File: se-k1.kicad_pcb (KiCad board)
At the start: 2 copper layers, 100 x 70 mm, 42 parts, among them J1 USB_C_Receptacle_USB2.0_14P, M1 MountingHole_2.7mm_M2.5, M2 MountingHole_2.7mm_M2.5, M3 MountingHole_2.7mm_M2.5, M4 MountingHole_2.7mm_M2.5, U1 ESP32-S3-MINI-1U, U3 W25Q16JVSSIQ, U4 AMS1117-3.3

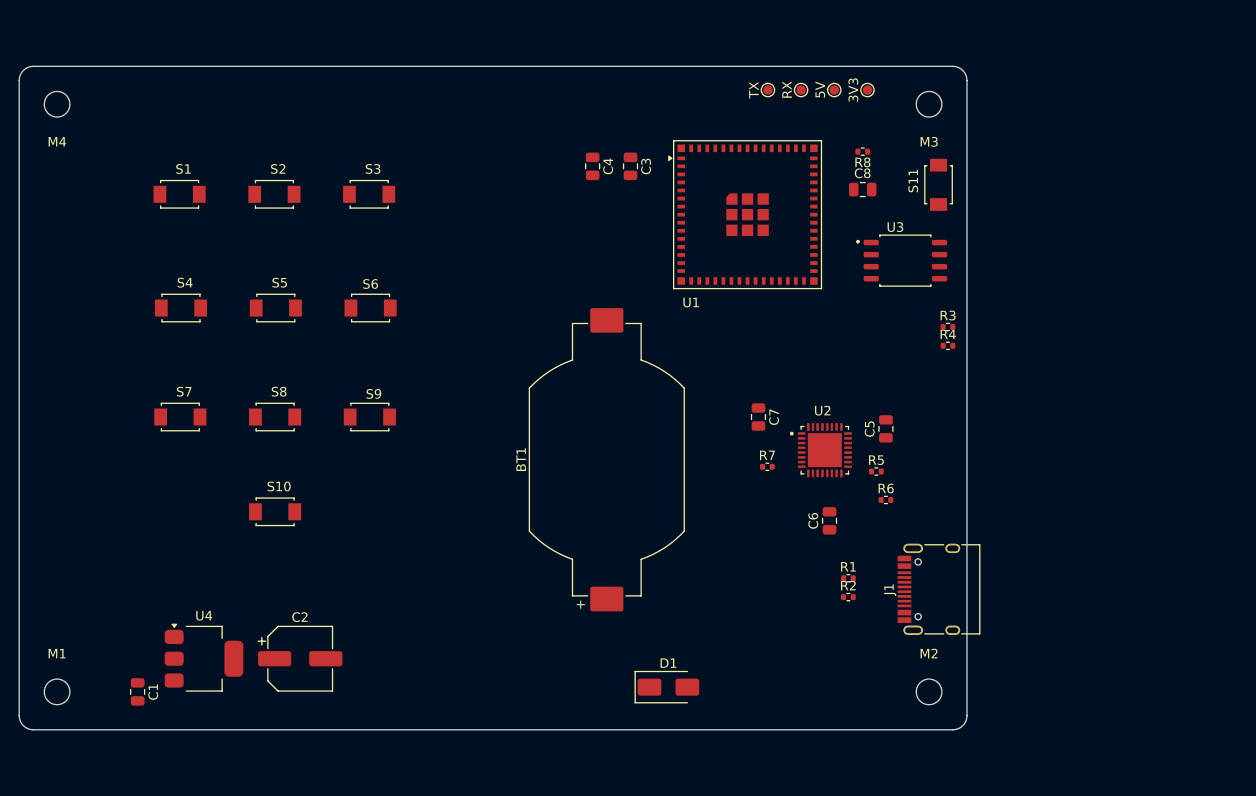
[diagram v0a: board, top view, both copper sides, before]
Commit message: finish!
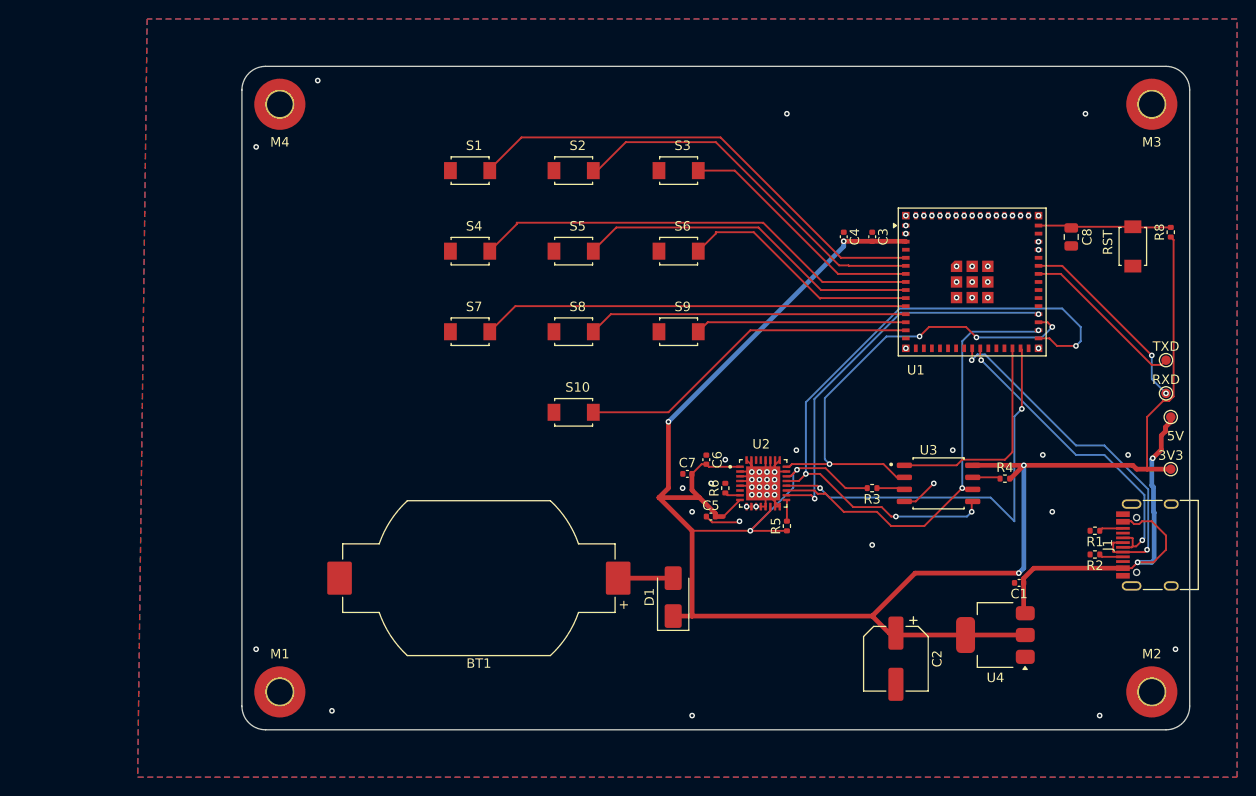
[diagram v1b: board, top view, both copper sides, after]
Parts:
- removed R7: 10k, Resistor_SMD:R_0402_1005Metric
- removed RX: RX, TestPoint:TestPoint_Pad_D1.0mm
- removed S11: TS-1088-AR02016, TS-1088-AR02016:SW_TS-1088-AR02016
- removed TX: TX, TestPoint:TestPoint_Pad_D1.0mm
- added RST: TS-1088-AR02016, TS-1088-AR02016:SW_TS-1088-AR02016, F.Cu at (194.0, 69.0)
- added RXD: RX, TestPoint:TestPoint_Pad_D1.0mm, F.Cu at (197.5, 84.5)
- added TXD: TX, TestPoint:TestPoint_Pad_D1.0mm, F.Cu at (197.5, 81.0)
- C1, C3, C4, C5, C6: footprint Capacitor_SMD:C_0805_2012Metric -> Capacitor_SMD:C_0402_1005Metric
- C7: value 100nF -> 10uF; footprint Capacitor_SMD:C_0805_2012Metric -> Capacitor_SMD:C_0402_1005Metric
- M1, M2, M3, M4: value MountingHole_2.7mm_M2.5 -> MountingHole_2.7mm_M2.5_Pad_TopOnly; footprint MountingHole:MountingHole_2.7mm_M2.5 -> MountingHole:MountingHole_2.7mm_M2.5_Pad_TopOnly
- U2: value ~ -> SLM9670AQ20FW1311XTMA1; footprint SLB9670VQ20FW785XUMA1:QFN50P500X500X90-33N -> SLM9670AQ20FW1311XTMA1:QFN50P500X500X90-33N
- moved C1 93.7 mm to (182.0, 104.5), turned to 180 degrees
- moved U4 83.5 mm to (179.5, 110.0), turned to 180 degrees
- moved C2 62.8 mm to (169.0, 112.5), turned to -90 degrees
- moved 3V3 51.2 mm to (198.0, 92.5), turned to 0 degrees
- moved 5V 49.5 mm to (198.0, 87.0), turned to 0 degrees
- moved S9 33.8 mm to (146.1, 78.0)
- moved R8 33.6 mm to (198.0, 67.5), turned to 90 degrees
- moved S10 33.2 mm to (135.0, 86.5)
- moved S6 33.0 mm to (146.1, 69.5)
- moved S8 32.8 mm to (135.0, 78.0)
- moved S3 32.7 mm to (146.1, 61.0)
- moved S5 32.0 mm to (135.0, 69.5)
- moved S7 31.9 mm to (124.1, 78.0)
- moved S2 31.7 mm to (135.0, 61.0)
- moved S4 31.1 mm to (124.1, 69.5)
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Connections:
- C5 pad 1: +3V3 -> GND
- C5 pad 2: GND -> +3V3
- R5 pad 1: /TPM_PIRQ -> +3V3
- R5 pad 2: +3V3 -> Net-(U2-~{RST})
- R6 pad 1: Net-(U2-RST) -> Net-(U2-PP)
- R6 pad 2: +3V3 -> GND
- S2 pad 2: /B4 -> /B2
- S3 pad 2: /B7 -> /B3
- S6 pad 2: /B8 -> /B6
- S7 pad 2: /B3 -> /B7
- S8 pad 2: /B6 -> /B8
- U2 pad 10: unconnected-(U2-NC-Pad10) -> GND
- U2 pad 11: unconnected-(U2-NC-Pad11) -> GND
- U2 pad 12: unconnected-(U2-NC-Pad12) -> GND
- U2 pad 13: unconnected-(U2-NC-Pad13) -> GND
- U2 pad 15: unconnected-(U2-NC-Pad15) -> GND
- U2 pad 17: Net-(U2-RST) -> Net-(U2-~{RST})
- U2 pad 25: unconnected-(U2-NC-Pad25) -> GND
- U2 pad 26: unconnected-(U2-NC-Pad26) -> GND
- U2 pad 27: unconnected-(U2-NC-Pad27) -> GND
- U2 pad 28: unconnected-(U2-NC-Pad28) -> GND
- U2 pad 29: unconnected-(U2-NC-Pad29) -> (no net)
- U2 pad 3: unconnected-(U2-NC-Pad3) -> GND
- U2 pad 30: unconnected-(U2-NC-Pad30) -> (no net)
- U2 pad 31: unconnected-(U2-NC-Pad31) -> GND
- U2 pad 33: (no net) -> GND
- U2 pad 4: unconnected-(U2-NC-Pad4) -> GND
- U2 pad 5: unconnected-(U2-NC-Pad5) -> GND
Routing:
- net +3V3: track 0.00 -> 222.2 mm, vias 0 -> 6
- net /MOSI: track 0.00 -> 71.0 mm, vias 0 -> 4
- net /B1: track 0.00 -> 50.7 mm
- net /MISO: track 0.00 -> 50.0 mm, vias 0 -> 4
- net /B4: track 0.00 -> 47.8 mm
- net /SCLK: track 0.00 -> 47.0 mm, vias 0 -> 2
- net /B7: track 0.00 -> 45.0 mm
- net +5V: track 0.00 -> 44.8 mm, vias 0 -> 2
- net /TPM_CS: track 0.00 -> 44.2 mm, vias 0 -> 2
- net /TPM_PIRQ: track 0.00 -> 41.1 mm, vias 0 -> 2
- net GND: track 0.00 -> 39.7 mm, vias 0 -> 71
- net /B2: track 0.00 -> 39.6 mm
- net /D-: track 0.00 -> 38.1 mm, vias 0 -> 2
- net /B5: track 0.00 -> 36.8 mm
- net /B0: track 0.00 -> 36.6 mm
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- added copper zone on B.Cu, net GND
- added copper zone on F.Cu, net GND
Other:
- outline, holes or cut-outs redrawn
